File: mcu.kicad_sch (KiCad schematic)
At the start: 5 parts, among them U1 MIMXRT1052CVJ5B

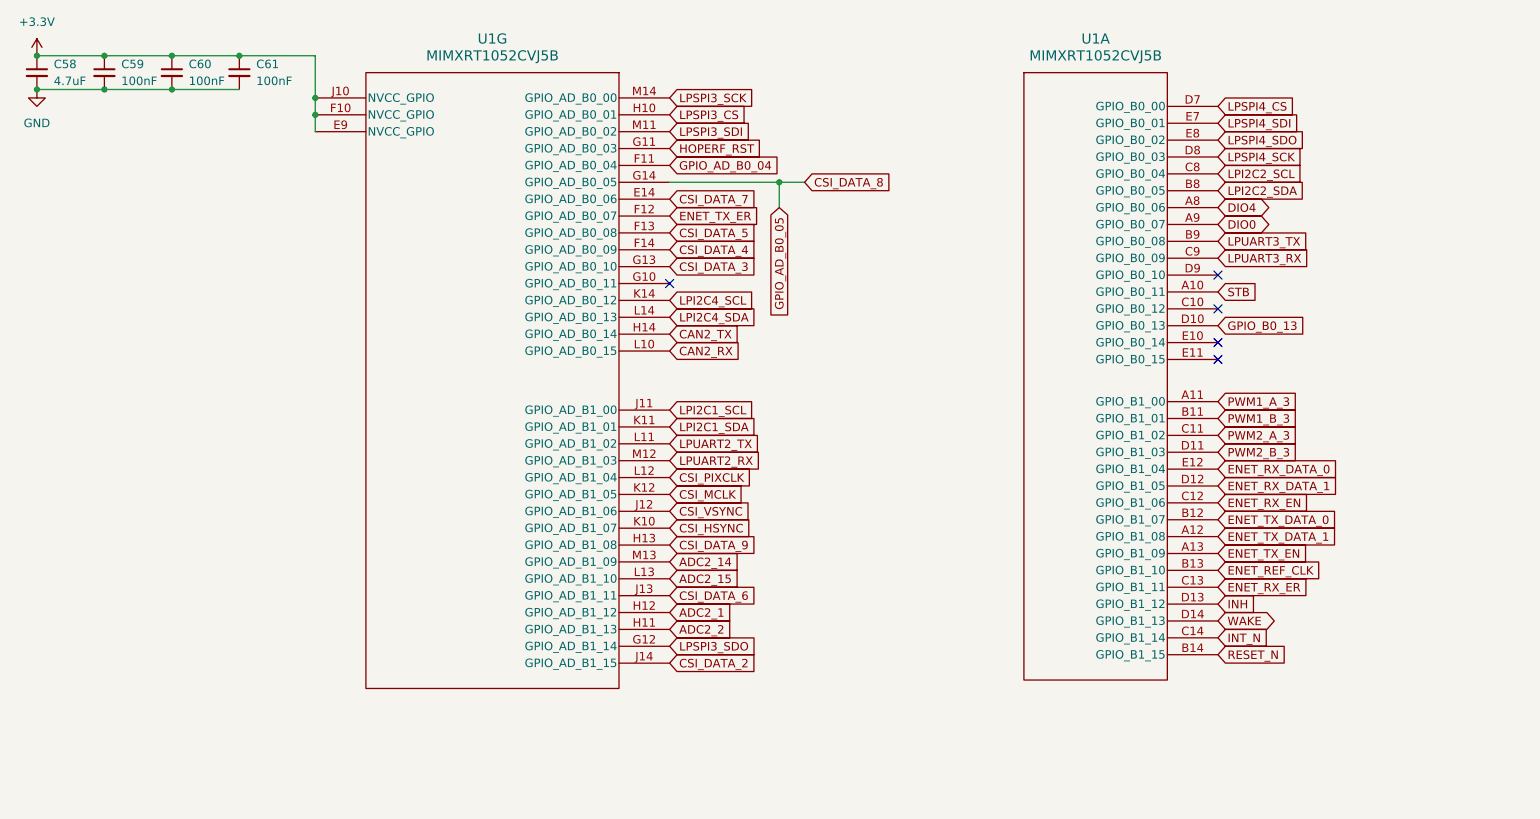
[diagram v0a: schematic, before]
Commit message: v0.2
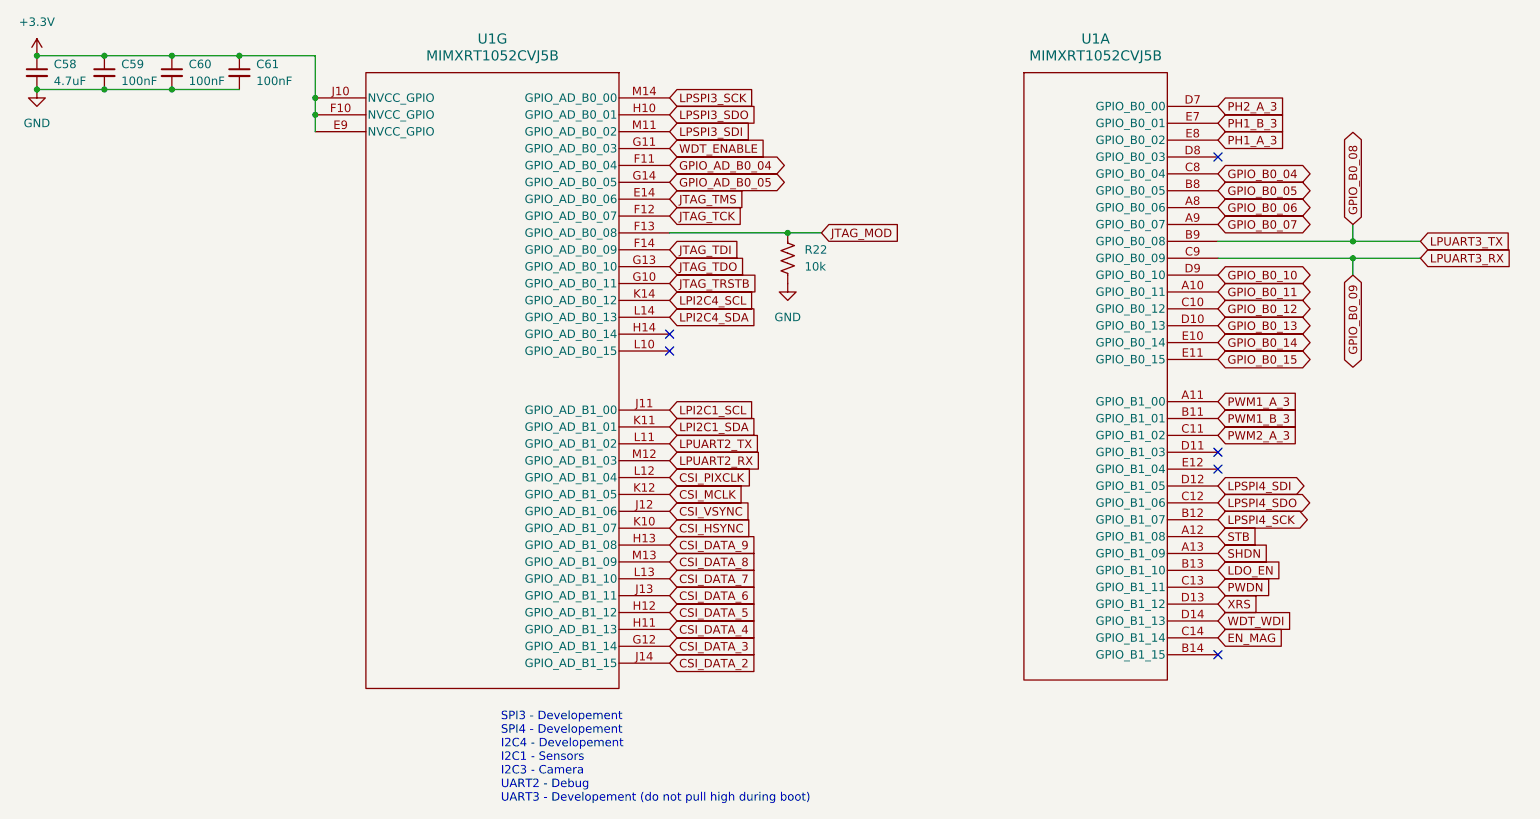
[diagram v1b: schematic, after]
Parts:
- added R22: 10k, symbol Device:R_US
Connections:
- net ADC2_1 is gone; now on net CSI_DATA_5: U1.H12 (GPIO_AD_B1_12)
- net ADC2_14 is gone; now on net CSI_DATA_8: U1.M13 (GPIO_AD_B1_09)
- net ADC2_15 is gone; now on net CSI_DATA_7: U1.L13 (GPIO_AD_B1_10)
- net ADC2_2 is gone; now on net CSI_DATA_4: U1.H11 (GPIO_AD_B1_13)
- net ENET_RX_DATA_1 is gone; now on net LPSPI4_SDI: U1.D12 (GPIO_B1_05)
- net ENET_RX_EN is gone; now on net LPSPI4_SDO: U1.C12 (GPIO_B1_06)
- net ENET_TX_DATA_0 is gone; now on net LPSPI4_SCK: U1.B12 (GPIO_B1_07)
- net ENET_TX_DATA_1 is gone; now on net STB: U1.A12 (GPIO_B1_08)
- net LPSPI3_CS is gone; now on net LPSPI3_SDO: U1.H10 (GPIO_AD_B0_01)
- net CSI_DATA_3: now also U1.G12 (GPIO_AD_B1_14); no longer U1.G13 (GPIO_AD_B0_10)
- net CSI_DATA_4: no longer U1.F14 (GPIO_AD_B0_09)
- net CSI_DATA_5: no longer U1.F13 (GPIO_AD_B0_08)
- net CSI_DATA_7: no longer U1.E14 (GPIO_AD_B0_06)
- net CSI_DATA_8: no longer U1.G14 (GPIO_AD_B0_05)
- net GND: now also R22.2
- net LPSPI3_SDO: no longer U1.G12 (GPIO_AD_B1_14)
- net LPSPI4_SCK: no longer U1.D8 (GPIO_B0_03)
- net LPSPI4_SDI: no longer U1.E7 (GPIO_B0_01)
- net LPSPI4_SDO: no longer U1.E8 (GPIO_B0_02)
- net STB: no longer U1.A10 (GPIO_B0_11)
- net JTAG_TRSTB: now reaches U1.G10 (GPIO_AD_B0_11)
- net GPIO_B0_12: now reaches U1.C10 (GPIO_B0_12)
- net GPIO_B0_10: now reaches U1.D9 (GPIO_B0_10)
- net GPIO_B0_14: now reaches U1.E10 (GPIO_B0_14)
- net GPIO_B0_15: now reaches U1.E11 (GPIO_B0_15)
- net CAN2_RX: no longer names the net of U1.L10 (GPIO_AD_B0_15)
- net CAN2_TX: no longer names the net of U1.H14 (GPIO_AD_B0_14)
- net DIO0 renamed GPIO_B0_07
- net DIO4 renamed GPIO_B0_06
- net ENET_REF_CLK renamed LDO_EN
- net ENET_RX_DATA_0: no longer names the net of U1.E12 (GPIO_B1_04)
- net ENET_RX_ER renamed PWDN
- net ENET_TX_EN renamed SHDN
- net ENET_TX_ER renamed JTAG_TCK
- net HOPERF_RST renamed WDT_ENABLE
- net INH renamed XRS
- net INT_N renamed EN_MAG
- net LPI2C2_SCL renamed GPIO_B0_04
- net LPI2C2_SDA renamed GPIO_B0_05
- net LPSPI4_CS renamed PH2_A_3
- net LPUART3_RX renamed GPIO_B0_09
- net LPUART3_TX renamed GPIO_B0_08
- net PWM2_B_3: no longer names the net of U1.D11 (GPIO_B1_03)
- net RESET_N: no longer names the net of U1.B14 (GPIO_B1_15)
- net WAKE renamed WDT_WDI
- new net GPIO_AD_B0_05: U1.G14 (GPIO_AD_B0_05)
- new net GPIO_B0_11: U1.A10 (GPIO_B0_11)
- new net JTAG_MOD: R22.1, U1.F13 (GPIO_AD_B0_08)
- new net JTAG_TDI: U1.F14 (GPIO_AD_B0_09)
- new net JTAG_TDO: U1.G13 (GPIO_AD_B0_10)
- new net JTAG_TMS: U1.E14 (GPIO_AD_B0_06)
- new net PH1_A_3: U1.E8 (GPIO_B0_02)
- new net PH1_B_3: U1.E7 (GPIO_B0_01)
- no-connect marks 5 -> 6
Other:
- note added: "SPI3 - Developement SPI4 - Developement I2C4 - Developement I2C1 - Sensors I2C3 - Camera UART2 - Debug UART3 - Developement (do not pull high during boot)"
- title: RT1050 DevBoard for Project Horizon -> Payload Board for Pleiades Atlas
